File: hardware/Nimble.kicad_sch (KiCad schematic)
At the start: 14 parts, among them J1 TYPE-C-31-M-12, J3 Conn_01x16_Socket, SW1 Slideswitch, U1 W65C02SxP, U2 74HC00, U3 IS62C256AL-45ULI, U4 AT28C256-15PU, U5 W65C22SxP, Y1 ECS-10-13-1XH

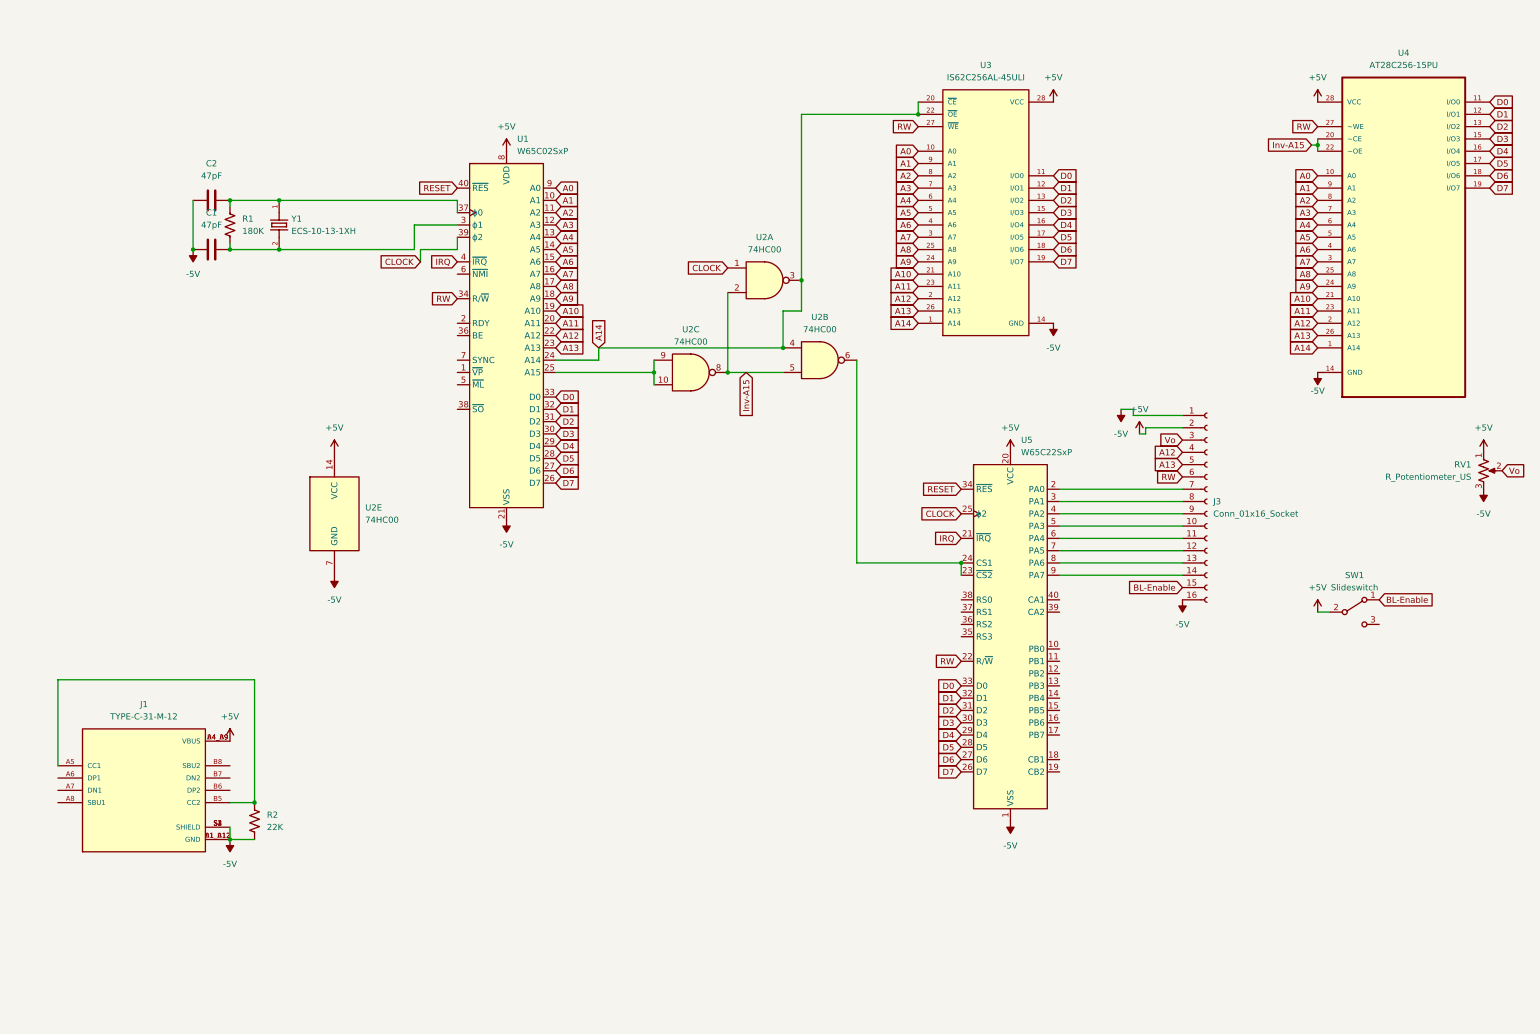
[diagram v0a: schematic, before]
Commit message: added hardware so far
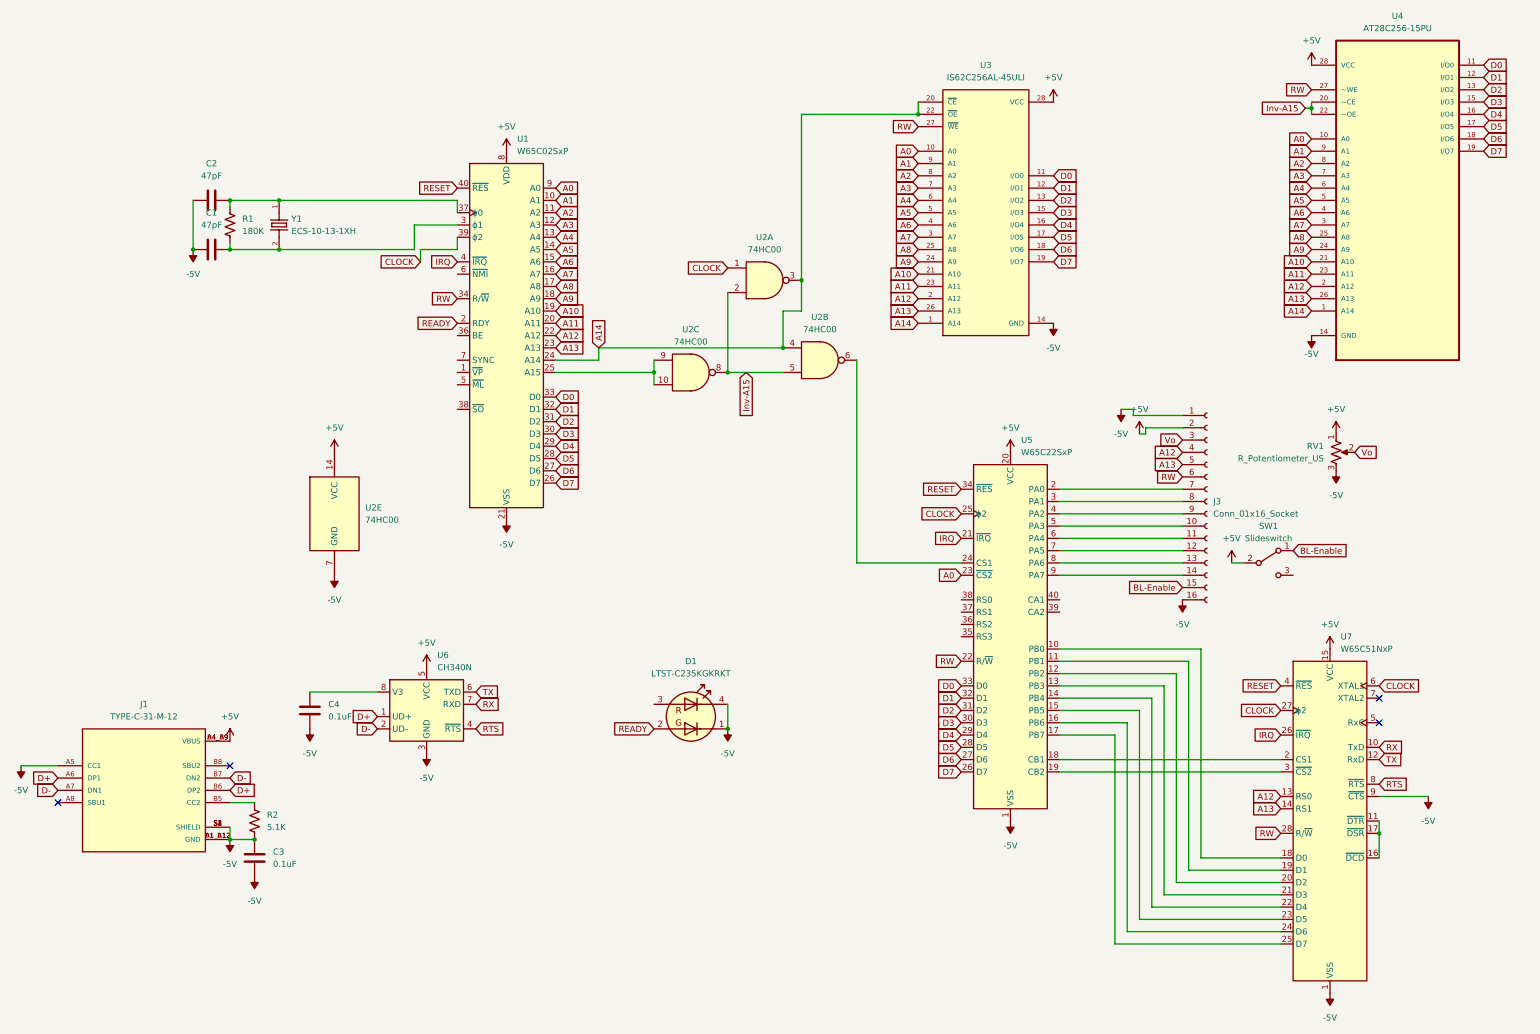
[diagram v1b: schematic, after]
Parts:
- added C3, C4: 0.1uF, symbol Device:C
- added D1: LTST-C235KGKRKT, LED_SMD:LED_LiteOn_LTST-C235KGKRKT, symbol LED:LTST-C235KGKRKT
- added U6: CH340N, Package_SO:SOP-8_3.9x4.9mm_P1.27mm, symbol Interface_USB:CH340N
- added U7: W65C51NxP, Package_DIP:DIP-28_W15.24mm, symbol PCM_65xx-library:W65C51NxP
- R2: value 22K -> 5.1K
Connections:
- net +5V: now also U6.5 (VCC), U7.15 (VCC)
- net -5V: now also J1.A5 (CC1), C3.1, C3.2, C4.2, D1.1 (K2), D1.4 (K1), U6.3 (GND), U7.1 (VSS), U7.9 (~{CTS})
- net A0: now also U5.23 (~{CS2})
- net A12: now also U7.13 (RS0)
- net A13: now also U7.14 (RS1)
- net CLOCK: now also U7.27 (ϕ2), U7.6 (XTAL1)
- net IRQ: now also U7.26 (~{IRQ})
- net RESET: now also U7.4 (~{RES})
- net RW: now also U7.28 (R/~{W})
- net at J1.B5 (CC2), R2.1: no longer J1.A5 (CC1)
- net at U2.6, U5.24 (CS1): no longer U5.23 (~{CS2})
- net D+: now reaches J1.A6 (DP1)
- net D+: now also J1.B6 (DP2), U6.1 (UD+)
- net D-: now reaches J1.A7 (DN1)
- net D-: now also J1.B7 (DN2), U6.2 (UD-)
- net at U5.10 (PB0): now also U7.18 (D0)
- net at U5.11 (PB1): now also U7.19 (D1)
- net at U5.12 (PB2): now also U7.20 (D2)
- net at U5.13 (PB3): now also U7.21 (D3)
- net at U5.14 (PB4): now also U7.22 (D4)
- net at U5.15 (PB5): now also U7.23 (D5)
- net at U5.16 (PB6): now also U7.24 (D6)
- net at U5.17 (PB7): now also U7.25 (D7)
- net at U5.18 (CB1): now also U7.2 (CS1)
- net at U5.19 (CB2): now also U7.3 (~{CS2})
- net READY: now reaches U1.2 (RDY)
- net READY: now also D1.2 (A2)
- new net: C4.1, U6.8 (V3)
- new net: U7.11 (~{DTR}), U7.16 (~{DCD}), U7.17 (~{DSR})
- new net RTS: U6.4 (~{RTS}), U7.8 (~{RTS})
- new net RX: U6.7 (RXD), U7.10 (TxD)
- new net TX: U6.6 (TXD), U7.12 (RxD)
- no-connect marks 0 -> 4
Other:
- moved on the sheet: RV1, SW1, U4

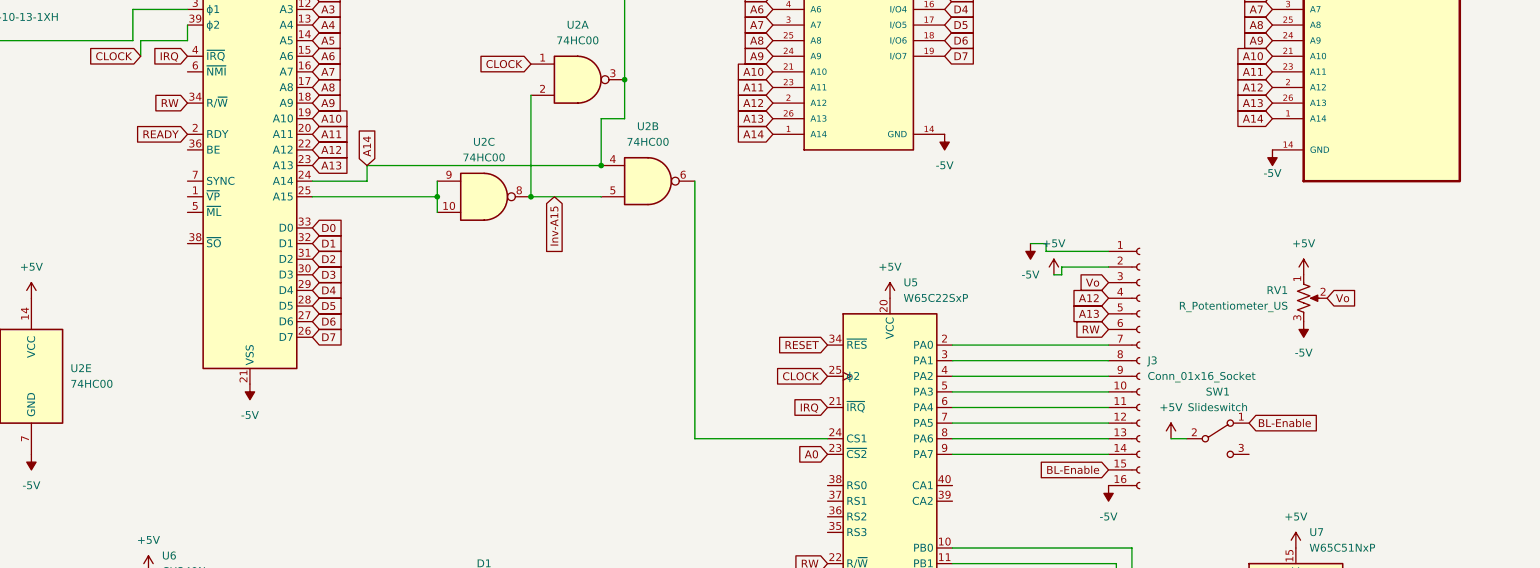
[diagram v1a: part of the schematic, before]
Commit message: hardware upload so far
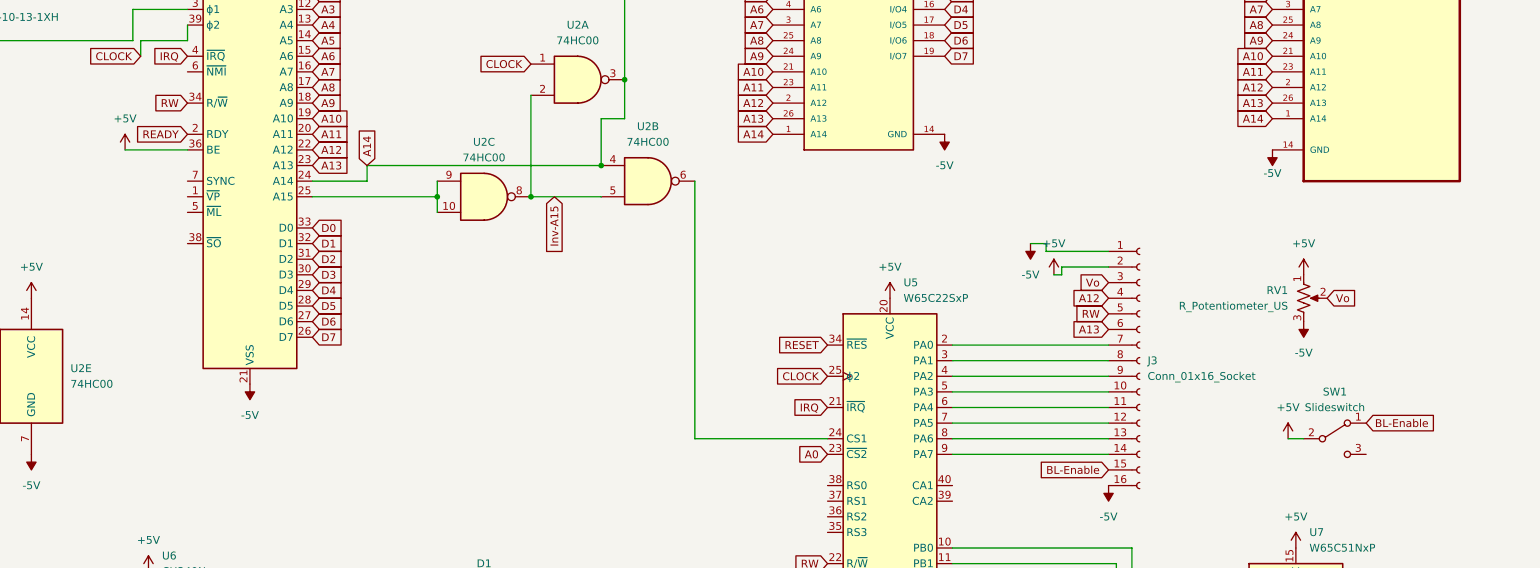
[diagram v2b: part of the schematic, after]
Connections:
- net +5V: now also U1.36 (BE)
- net A13: now also J3.6 (Pin_6); no longer J3.5 (Pin_5)
- net RW: now also J3.5 (Pin_5); no longer J3.6 (Pin_6)
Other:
- moved on the sheet: SW1
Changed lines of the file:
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@@
 	(wire
 		(pts
+			(xy 97.79 92.71) (xy 107.95 92.71)
+		)
+		(stroke
+			(width 0)
+			(type default)
+		)
+	)
+	(wire
+		(pts
 			(xy 232.41 172.72) (xy 246.38 172.72)
 		)
@@
 	(wire
 		(pts
-			(xy 267.97 139.7) (xy 270.51 139.7)
+			(xy 287.02 139.7) (xy 289.56 139.7)
 		)
 		(stroke
@@
 		)
 	)
-	(global_label "RW"
+	(global_label "TX"
 		(shape input)
-		(at 257.81 121.92 180)
+		(at 111.76 166.37 0)
 		(fields_autoplaced yes)
 		(effects
@@
 				(size 1.27 1.27)
 			)
-			(justify right)
+			(justify left)
 		)
 		(property "Intersheetrefs" "${INTERSHEET_REFS}"
-			(at 252.1034 121.92 0)
+			(at 116.9223 166.37 0)
 			(effects
 				(font
 					(size 1.27 1.27)
 				)
-				(justify right)
+				(justify left)
 				(hide yes)
 			)
 		)
 	)
-	(global_label "TX"
+	(global_label "A5"
 		(shape input)
-		(at 111.76 166.37 0)
+		(at 128.27 74.93 0)
 		(fields_autoplaced yes)
 		(effects
@@
 		)
 		(property "Intersheetrefs" "${INTERSHEET_REFS}"
-			(at 116.9223 166.37 0)
+			(at 133.5533 74.93 0)
 			(effects
 				(font
@@
 		)
 	)
-	(global_label "A5"
+	(global_label "A13"
 		(shape input)
-		(at 128.27 74.93 0)
+		(at 257.81 121.92 180)
 		(fields_autoplaced yes)
 		(effects
@@
 				(size 1.27 1.27)
 			)
-			(justify left)
+			(justify right)
 		)
 		(property "Intersheetrefs" "${INTERSHEET_REFS}"
-			(at 133.5533 74.93 0)
+			(at 251.3172 121.92 0)
 			(effects
 				(font
 					(size 1.27 1.27)
 				)
-				(justify left)
+				(justify right)
 				(hide yes)
 			)
@@
 		)
 	)
+	(global_label "RW"
+		(shape input)
+		(at 257.81 119.38 180)
+		(fields_autoplaced yes)
+		(effects
+			(font
+				(size 1.27 1.27)
+			)
+			(justify right)
+		)
+		(property "Intersheetrefs" "${INTERSHEET_REFS}"
+			(at 252.1034 119.38 0)
+			(effects
+				(font
+					(size 1.27 1.27)
+				)
+				(justify right)
+				(hide yes)
+			)
+		)
+	)
 	(global_label "BL-Enable"
 		(shape input)
-		(at 280.67 137.16 0)
+		(at 299.72 137.16 0)
 		(fields_autoplaced yes)
 		(effects
@@
 		)
 		(property "Intersheetrefs" "${INTERSHEET_REFS}"
-			(at 293.8755 137.16 0)
+			(at 312.9255 137.16 0)
 			(effects
 				(font
@@
 		)
 	)
-	(global_label "A13"
-		(shape input)
-		(at 257.81 119.38 180)
-		(fields_autoplaced yes)
-		(effects
-			(font
-				(size 1.27 1.27)
-			)
-			(justify right)
-		)
-		(property "Intersheetrefs" "${INTERSHEET_REFS}"
-			(at 251.3172 119.38 0)
-			(effects
-				(font
-					(size 1.27 1.27)
-				)
-				(justify right)
-				(hide yes)
-			)
-		)
-	)
 	(global_label "D6"
 		(shape input)
@@
 	(symbol
 		(lib_id "fab:SWITCH_AYZ0102AGRLC")
-		(at 275.59 139.7 0)
+		(at 294.64 139.7 0)
 		(unit 1)
 		(exclude_from_sim no)
@@
 		(fields_autoplaced yes)
 		(property "Reference" "SW1"
-			(at 275.59 132.08 0)
+			(at 294.64 132.08 0)
 			(effects
 				(font
@@
 		)
 		(property "Value" "Slideswitch"
-			(at 275.59 134.62 0)
+			(at 294.64 134.62 0)
 			(effects
 				(font
@@
 		)
 		(property "Footprint" "slideSWSMD:slideswitchCK"
-			(at 275.59 139.7 0)
+			(at 294.64 139.7 0)
 			(effects
 				(font
@@
 		)
 		(property "Datasheet" "https://www.ckswitches.com/media/1431/ayz.pdf"
-			(at 275.59 139.7 0)
+			(at 294.64 139.7 0)
 			(effects
 				(font
@@
 		)
 		(property "Description" ""
-			(at 275.59 139.7 0)
+			(at 294.64 139.7 0)
 			(effects
 				(font
@@
 	(symbol
 		(lib_id "power:+5V")
-		(at 267.97 139.7 0)
+		(at 287.02 139.7 0)
 		(unit 1)
 		(exclude_from_sim no)
@@
 		(fields_autoplaced yes)
 		(property "Reference" "#PWR021"
-			(at 267.97 143.51 0)
+			(at 287.02 143.51 0)
 			(effects
 				(font
@@
 		)
 		(property "Value" "+5V"
-			(at 267.97 134.62 0)
+			(at 287.02 134.62 0)
 			(effects
 				(font
@@
 		)
 		(property "Footprint" ""
-			(at 267.97 139.7 0)
+			(at 287.02 139.7 0)
 			(effects
 				(font
@@
 		)
 		(property "Datasheet" ""
-			(at 267.97 139.7 0)
+			(at 287.02 139.7 0)
 			(effects
 				(font
@@
 		)
 		(property "Description" "Power symbol creates a global label with name \"+5V\""
-			(at 267.97 139.7 0)
+			(at 287.02 139.7 0)
 			(effects
 				(font
@@
 					(unit 1)
 				)
+			)
+		)
+	)
+	(symbol
+		(lib_id "power:+5V")
+		(at 97.79 92.71 0)
+		(unit 1)
+		(exclude_from_sim no)
+		(in_bom yes)
+		(on_board yes)
+		(dnp no)
+		(fields_autoplaced yes)
+		(property "Reference" "#PWR029"
+			(at 97.79 96.52 0)
+			(effects
+				(font
+					(size 1.27 1.27)
+				)
+				(hide yes)
+			)
+		)
+		(property "Value" "+5V"
+			(at 97.79 87.63 0)
+			(effects
+				(font
+					(size 1.27 1.27)
+				)
+			)
+		)
+		(property "Footprint" ""
+			(at 97.79 92.71 0)
+			(effects
+				(font
+					(size 1.27 1.27)
+				)
+				(hide yes)
+			)
+		)
+		(property "Datasheet" ""
+			(at 97.79 92.71 0)
+			(effects
+				(font
+					(size 1.27 1.27)
+				)
+				(hide yes)
+			)
+		)
+		(property "Description" "Power symbol creates a global label with name \"+5V\""
+			(at 97.79 92.71 0)
+			(effects
+				(font
+					(size 1.27 1.27)
+				)
+				(hide yes)
+			)
+		)
+		(pin "1"
+		)
+		(instances
+			(project "Nimble"
+				(path "/cac1b442-1e9b-4849-bc2f-933ec367e12a"
+					(reference "#PWR029")
+					(unit 1)
+				)
